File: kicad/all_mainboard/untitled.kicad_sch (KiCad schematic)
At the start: 136 parts, among them SW1 SW_Push, SW10 SW_Push, SW11 SW_Push, SW12 SW_Push, SW13 SW_Push, SW14 SW_Push, SW15 SW_Push, SW16 SW_Push, SW17 SW_Push, SW18 SW_Push, SW19 SW_Push, SW2 SW_Push, SW20 SW_Push, SW21 SW_Push, SW22 SW_Push, SW23 SW_Push, SW24 SW_Push, SW25 SW_Push, SW26 SW_Push, SW27 SW_Push, SW28 SW_Push, SW29 SW_Push, SW3 SW_Push, SW30 SW_Push, SW31 SW_Push, SW32 SW_Push, SW33 SW_Push, SW34 SW_Push, SW35 SW_Push, SW36 SW_Push, SW37 SW_Push, SW38 SW_Push, SW39 SW_Push, SW4 SW_Push, SW40 SW_Push, SW41 SW_Push, SW42 SW_Push, SW43 SW_Push, SW44 SW_Push, SW45 SW_Push, SW46 SW_Push, SW47 SW_Push, SW48 SW_Push, SW49 SW_Push, SW5 SW_Push, SW50 SW_Push, SW51 SW_Push, SW52 SW_Push, SW53 SW_Push, SW54 SW_Push, SW55 SW_Push, SW56 SW_Push, SW57 SW_Push, SW58 SW_Push, SW59 SW_Push, SW6 SW_Push, SW60 SW_Push, SW61 SW_Push, SW62 SW_Push, SW63 SW_Push, SW64 SW_Push, SW65 SW_Push, SW66 SW_Push, SW67 SW_Push, SW68 SW_Push, SW7 SW_Push, SW8 SW_Push, SW9 SW_Push

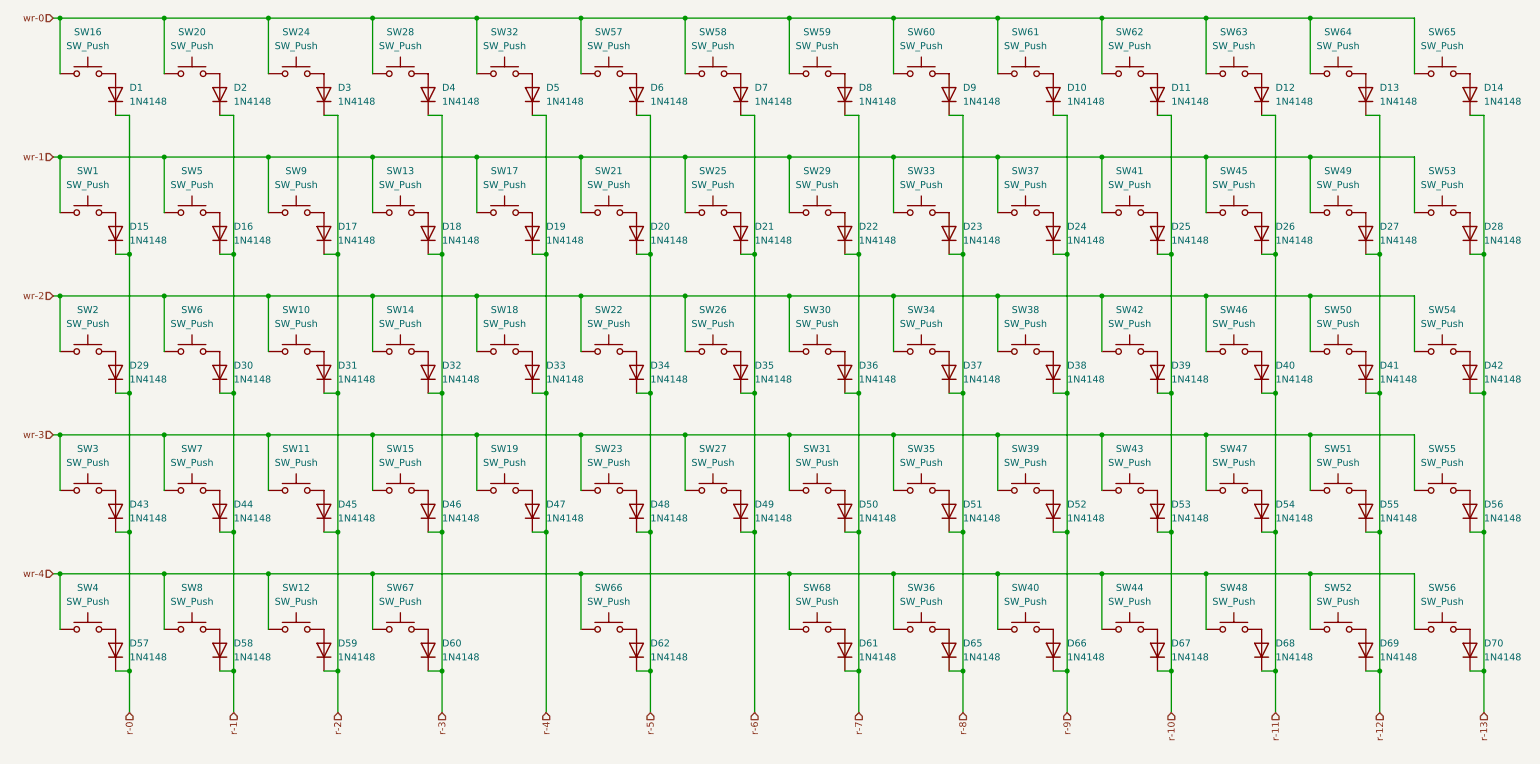
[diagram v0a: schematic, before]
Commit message: added kicad files
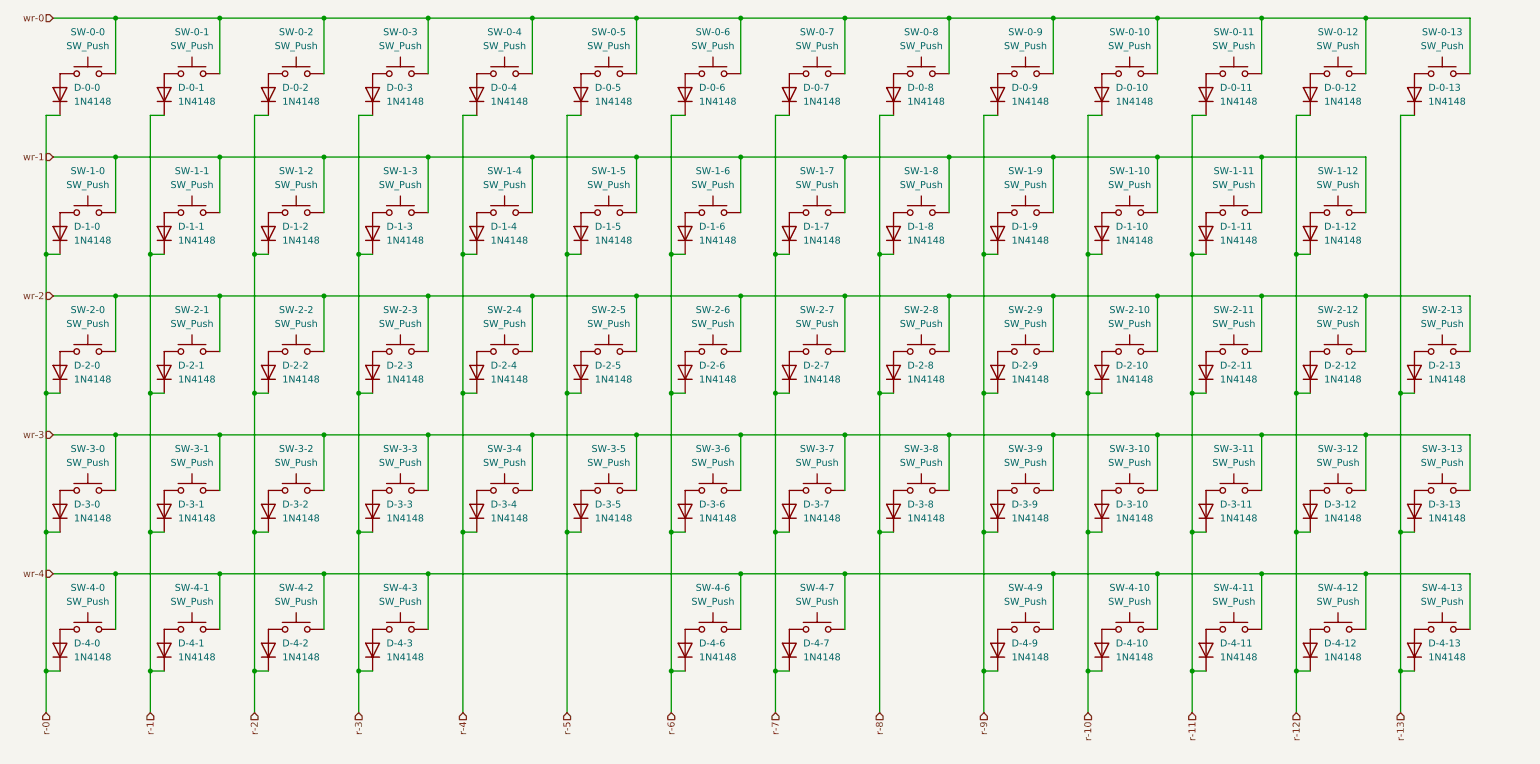
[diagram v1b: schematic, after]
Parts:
- removed D28, D61: 1N4148, Diode_THT:D_DO-35_SOD27_P7.62mm_Horizontal, symbol Diode:1N4148
- removed SW53, SW68: SW_Push, Button_Switch_Keyboard:SW_Cherry_MX_1.00u_PCB, symbol Switch:SW_Push
- renumbered D1 to D-0-0, D2 to D-0-1, D11 to D-0-10, D12 to D-0-11, D13 to D-0-12, D14 to D-0-13, D3 to D-0-2, D4 to D-0-3, D5 to D-0-4, D6 to D-0-5, D7 to D-0-6, D8 to D-0-7, D9 to D-0-8, D10 to D-0-9, D15 to D-1-0, D16 to D-1-1, D25 to D-1-10, D26 to D-1-11, D27 to D-1-12, D17 to D-1-2, D18 to D-1-3, D19 to D-1-4, D20 to D-1-5, D21 to D-1-6, D22 to D-1-7, D23 to D-1-8, D24 to D-1-9, D29 to D-2-0, D30 to D-2-1, D39 to D-2-10, D40 to D-2-11, D41 to D-2-12, D42 to D-2-13, D31 to D-2-2, D32 to D-2-3, D33 to D-2-4, D34 to D-2-5, D35 to D-2-6, D36 to D-2-7, D37 to D-2-8, D38 to D-2-9, D43 to D-3-0, D44 to D-3-1, D53 to D-3-10, D54 to D-3-11, D55 to D-3-12, D56 to D-3-13, D45 to D-3-2, D46 to D-3-3, D47 to D-3-4, D48 to D-3-5, D49 to D-3-6, D50 to D-3-7, D51 to D-3-8, D52 to D-3-9, D57 to D-4-0, D58 to D-4-1, D67 to D-4-10, D68 to D-4-11, D69 to D-4-12, D70 to D-4-13, D59 to D-4-2, D60 to D-4-3, D62 to D-4-6, D65 to D-4-7, D66 to D-4-9, SW16 to SW-0-0, SW20 to SW-0-1, SW62 to SW-0-10, SW63 to SW-0-11, SW64 to SW-0-12, SW65 to SW-0-13, SW24 to SW-0-2, SW28 to SW-0-3, SW32 to SW-0-4, SW57 to SW-0-5, SW58 to SW-0-6, SW59 to SW-0-7, SW60 to SW-0-8, SW61 to SW-0-9, SW1 to SW-1-0, SW5 to SW-1-1, SW41 to SW-1-10, SW45 to SW-1-11, SW49 to SW-1-12, SW9 to SW-1-2, SW13 to SW-1-3, SW17 to SW-1-4, SW21 to SW-1-5, SW25 to SW-1-6, SW29 to SW-1-7, SW33 to SW-1-8, SW37 to SW-1-9, SW2 to SW-2-0, SW6 to SW-2-1, SW42 to SW-2-10, SW46 to SW-2-11, SW50 to SW-2-12, SW54 to SW-2-13, SW10 to SW-2-2, SW14 to SW-2-3, SW18 to SW-2-4, SW22 to SW-2-5, SW26 to SW-2-6, SW30 to SW-2-7, SW34 to SW-2-8, SW38 to SW-2-9, SW3 to SW-3-0, SW7 to SW-3-1, SW43 to SW-3-10, SW47 to SW-3-11, SW51 to SW-3-12, SW55 to SW-3-13, SW11 to SW-3-2, SW15 to SW-3-3, SW19 to SW-3-4, SW23 to SW-3-5, SW27 to SW-3-6, SW31 to SW-3-7, SW35 to SW-3-8, SW39 to SW-3-9, SW4 to SW-4-0, SW8 to SW-4-1, SW44 to SW-4-10, SW48 to SW-4-11, SW52 to SW-4-12, SW56 to SW-4-13, SW12 to SW-4-2, SW67 to SW-4-3, SW66 to SW-4-6, SW36 to SW-4-7, SW40 to SW-4-9
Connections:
- net r-5: no longer D-4-6.1 (K)
- net r-6: now also D-4-6.1 (K)
- net r-7: now also D-4-7.1 (K)
- net r-8: no longer D-4-7.1 (K)
- net wr-0: now also SW-0-0.2, SW-0-1.2, SW-0-10.2, SW-0-11.2, SW-0-12.2, SW-0-13.2, SW-0-2.2, SW-0-3.2, SW-0-4.2, SW-0-5.2, SW-0-6.2, SW-0-7.2, SW-0-8.2, SW-0-9.2; no longer SW-0-0.1, SW-0-1.1, SW-0-10.1, SW-0-11.1, SW-0-12.1, SW-0-13.1, SW-0-2.1, SW-0-3.1, SW-0-4.1, SW-0-5.1, SW-0-6.1, SW-0-7.1, SW-0-8.1, SW-0-9.1
- net wr-1: now also SW-1-0.2, SW-1-1.2, SW-1-10.2, SW-1-11.2, SW-1-12.2, SW-1-2.2, SW-1-3.2, SW-1-4.2, SW-1-5.2, SW-1-6.2, SW-1-7.2, SW-1-8.2, SW-1-9.2; no longer SW-1-0.1, SW-1-1.1, SW-1-10.1, SW-1-11.1, SW-1-12.1, SW-1-2.1, SW-1-3.1, SW-1-4.1, SW-1-5.1, SW-1-6.1, SW-1-7.1, SW-1-8.1, SW-1-9.1
- net wr-2: now also SW-2-0.2, SW-2-1.2, SW-2-10.2, SW-2-11.2, SW-2-12.2, SW-2-13.2, SW-2-2.2, SW-2-3.2, SW-2-4.2, SW-2-5.2, SW-2-6.2, SW-2-7.2, SW-2-8.2, SW-2-9.2; no longer SW-2-0.1, SW-2-1.1, SW-2-10.1, SW-2-11.1, SW-2-12.1, SW-2-13.1, SW-2-2.1, SW-2-3.1, SW-2-4.1, SW-2-5.1, SW-2-6.1, SW-2-7.1, SW-2-8.1, SW-2-9.1
- net wr-3: now also SW-3-0.2, SW-3-1.2, SW-3-10.2, SW-3-11.2, SW-3-12.2, SW-3-13.2, SW-3-2.2, SW-3-3.2, SW-3-4.2, SW-3-5.2, SW-3-6.2, SW-3-7.2, SW-3-8.2, SW-3-9.2; no longer SW-3-0.1, SW-3-1.1, SW-3-10.1, SW-3-11.1, SW-3-12.1, SW-3-13.1, SW-3-2.1, SW-3-3.1, SW-3-4.1, SW-3-5.1, SW-3-6.1, SW-3-7.1, SW-3-8.1, SW-3-9.1
- net wr-4: now also SW-4-0.2, SW-4-1.2, SW-4-10.2, SW-4-11.2, SW-4-12.2, SW-4-13.2, SW-4-2.2, SW-4-3.2, SW-4-6.2, SW-4-7.2, SW-4-9.2; no longer SW-4-0.1, SW-4-1.1, SW-4-10.1, SW-4-11.1, SW-4-12.1, SW-4-13.1, SW-4-2.1, SW-4-3.1, SW-4-6.1, SW-4-7.1, SW-4-9.1
- net at D-2-9.2 (A): now also SW-2-9.1; no longer SW-2-9.2
- net at D-2-13.2 (A): now also SW-2-13.1; no longer SW-2-13.2
- net at D-0-12.2 (A): now also SW-0-12.1; no longer SW-0-12.2
- net at D-3-9.2 (A): now also SW-3-9.1; no longer SW-3-9.2
- net at D-4-7.2 (A): now also SW-4-7.1; no longer SW-4-7.2
- net at D-3-4.2 (A): now also SW-3-4.1; no longer SW-3-4.2
- net at D-3-12.2 (A): now also SW-3-12.1; no longer SW-3-12.2
- net at D-0-2.2 (A): now also SW-0-2.1; no longer SW-0-2.2
- net at D-0-5.2 (A): now also SW-0-5.1; no longer SW-0-5.2
- net at D-3-8.2 (A): now also SW-3-8.1; no longer SW-3-8.2
- net at D-1-8.2 (A): now also SW-1-8.1; no longer SW-1-8.2
- net at D-3-1.2 (A): now also SW-3-1.1; no longer SW-3-1.2
- net at D-3-13.2 (A): now also SW-3-13.1; no longer SW-3-13.2
- net at D-1-1.2 (A): now also SW-1-1.1; no longer SW-1-1.2
- net at D-2-12.2 (A): now also SW-2-12.1; no longer SW-2-12.2
- net at D-4-12.2 (A): now also SW-4-12.1; no longer SW-4-12.2
- net at D-1-3.2 (A): now also SW-1-3.1; no longer SW-1-3.2
- net at D-0-9.2 (A): now also SW-0-9.1; no longer SW-0-9.2
- net at D-0-3.2 (A): now also SW-0-3.1; no longer SW-0-3.2
- net at D-3-0.2 (A): now also SW-3-0.1; no longer SW-3-0.2
- net at D-0-13.2 (A): now also SW-0-13.1; no longer SW-0-13.2
- net at D-4-0.2 (A): now also SW-4-0.1; no longer SW-4-0.2
- net at D-0-6.2 (A): now also SW-0-6.1; no longer SW-0-6.2
- net at D-3-5.2 (A): now also SW-3-5.1; no longer SW-3-5.2
- net at D-4-1.2 (A): now also SW-4-1.1; no longer SW-4-1.2
- net at D-0-11.2 (A): now also SW-0-11.1; no longer SW-0-11.2
- net at D-1-4.2 (A): now also SW-1-4.1; no longer SW-1-4.2
- net at D-0-10.2 (A): now also SW-0-10.1; no longer SW-0-10.2
- net at D-3-6.2 (A): now also SW-3-6.1; no longer SW-3-6.2
- net at D-2-10.2 (A): now also SW-2-10.1; no longer SW-2-10.2
- net at D-4-2.2 (A): now also SW-4-2.1; no longer SW-4-2.2
- net at D-0-0.2 (A): now also SW-0-0.1; no longer SW-0-0.2
- net at D-2-6.2 (A): now also SW-2-6.1; no longer SW-2-6.2
- net at D-4-6.2 (A): now also SW-4-6.1; no longer SW-4-6.2
- net at D-2-11.2 (A): now also SW-2-11.1; no longer SW-2-11.2
- net at D-3-7.2 (A): now also SW-3-7.1; no longer SW-3-7.2
- net at D-3-2.2 (A): now also SW-3-2.1; no longer SW-3-2.2
- net at D-0-8.2 (A): now also SW-0-8.1; no longer SW-0-8.2
- net at D-2-8.2 (A): now also SW-2-8.1; no longer SW-2-8.2
- net at D-2-3.2 (A): now also SW-2-3.1; no longer SW-2-3.2
- net at D-1-12.2 (A): now also SW-1-12.1; no longer SW-1-12.2
- net at D-0-4.2 (A): now also SW-0-4.1; no longer SW-0-4.2
- net at D-1-9.2 (A): now also SW-1-9.1; no longer SW-1-9.2
- net at D-4-3.2 (A): now also SW-4-3.1; no longer SW-4-3.2
- net at D-1-11.2 (A): now also SW-1-11.1; no longer SW-1-11.2
- net at D-0-1.2 (A): now also SW-0-1.1; no longer SW-0-1.2
- net at D-3-3.2 (A): now also SW-3-3.1; no longer SW-3-3.2
- net at D-1-10.2 (A): now also SW-1-10.1; no longer SW-1-10.2
- net at D-4-9.2 (A): now also SW-4-9.1; no longer SW-4-9.2
- net at D-4-10.2 (A): now also SW-4-10.1; no longer SW-4-10.2
- net at D-1-0.2 (A): now also SW-1-0.1; no longer SW-1-0.2
- net at D-2-5.2 (A): now also SW-2-5.1; no longer SW-2-5.2
- net at D-2-2.2 (A): now also SW-2-2.1; no longer SW-2-2.2
- net at D-4-13.2 (A): now also SW-4-13.1; no longer SW-4-13.2
- net at D-2-7.2 (A): now also SW-2-7.1; no longer SW-2-7.2
- net at D-2-1.2 (A): now also SW-2-1.1; no longer SW-2-1.2
- net at D-3-10.2 (A): now also SW-3-10.1; no longer SW-3-10.2
- net at D-1-6.2 (A): now also SW-1-6.1; no longer SW-1-6.2
- net at D-1-5.2 (A): now also SW-1-5.1; no longer SW-1-5.2
- net at D-1-7.2 (A): now also SW-1-7.1; no longer SW-1-7.2
- net at D-2-4.2 (A): now also SW-2-4.1; no longer SW-2-4.2
- net at D-0-7.2 (A): now also SW-0-7.1; no longer SW-0-7.2
- net at D-2-0.2 (A): now also SW-2-0.1; no longer SW-2-0.2
- net at D-3-11.2 (A): now also SW-3-11.1; no longer SW-3-11.2
- net at D-4-11.2 (A): now also SW-4-11.1; no longer SW-4-11.2
- net at D-1-2.2 (A): now also SW-1-2.1; no longer SW-1-2.2
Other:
- moved on the sheet: D-0-0, D-0-1, D-0-10, D-0-11, D-0-12, D-0-13, D-0-2, D-0-3, D-0-4, D-0-5, D-0-6, D-0-7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
